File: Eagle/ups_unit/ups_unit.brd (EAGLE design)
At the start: 61 x 20.3 mm, 36 parts

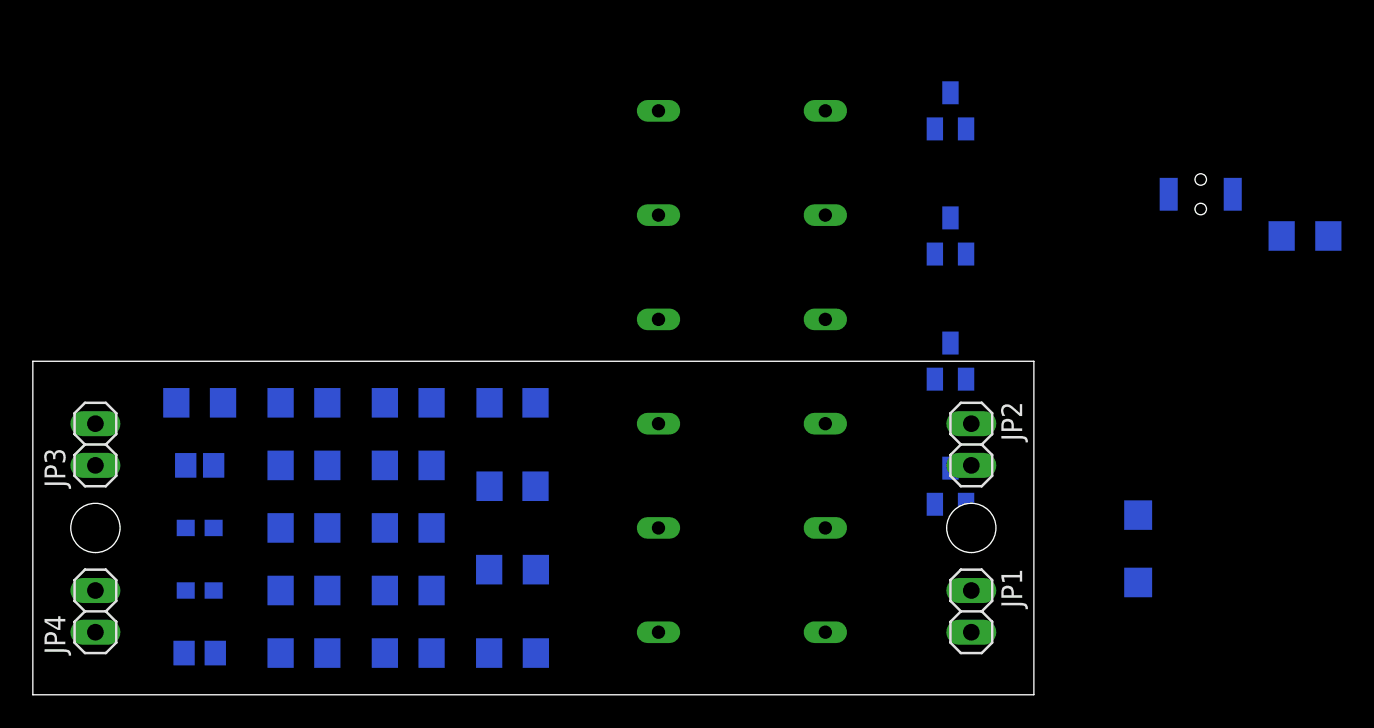
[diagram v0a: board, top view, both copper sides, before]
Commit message: RPi UPS unit
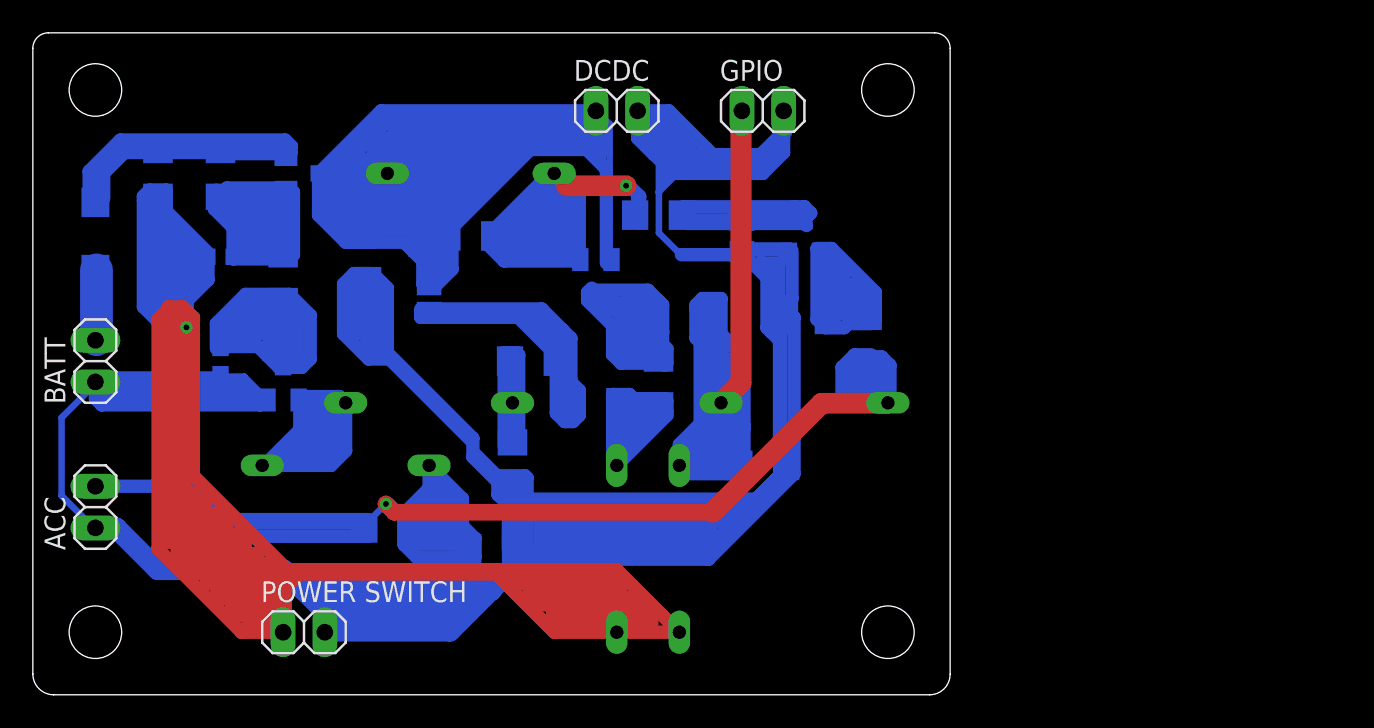
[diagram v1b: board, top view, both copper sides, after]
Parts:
- removed JP1, JP2, JP3, JP4: (no value), pinhead:1X02
- removed S1: MOMENTARY-SWITCH-SPST-SMD-RIGHT-ANGLE, SparkFun-Switches:TACTILE_SWITCH_SMD_RIGHT_ANGLE
- added ACC, BATT, DCDC, GPIO: (no value), pinhead:1X02
- added POWER　SWITCH: (no value), pinhead:1X02
- moved D9 66.3 mm to (3.81, 27.9)
- moved 22UF1 41.7 mm to (43.2, 27.9), turned to 270 degrees
- moved 2N7002K1 40.7 mm to (15.2, 19.1)
- moved DMG3415U2 39.6 mm to (16.5, 31.8), turned to 90 degrees
- moved 3.3K1 36.6 mm to (47.0, 22.9), turned to 180 degrees
- moved D1 32.4 mm to (19.1, 14.0), turned to 180 degrees
- moved 10K3 32.4 mm to (7.62, 31.8), turned to 90 degrees
- moved 5.6K1 29.6 mm to (39.4, 22.9)
- moved 1.8K1 29.0 mm to (44.5, 14.0)
- moved 5.6K2 27.4 mm to (50.8, 21.6), turned to 90 degrees
- moved 10K4 26.8 mm to (15.2, 25.4), turned to 90 degrees
- moved 100K1 24.4 mm to (11.4, 31.8), turned to 90 degrees
- moved DMG3415U1 21.7 mm to (34.3, 25.4), turned to 180 degrees
- moved 100K4 21.6 mm to (38.1, 19.1), turned to 90 degrees
- moved 10K6 21.6 mm to (38.1, 29.2)
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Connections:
- net ACC: now also ACC.2; no longer JP4.2
- net BATT: now also BATT.2; no longer JP3.2
- net DCDC: now also DCDC.1; no longer JP2.1
- net GND: now also ACC.1, BATT.1, DCDC.2, GPIO.2, POWER　SWITCH.2; no longer JP1.2, JP2.2, JP3.1, JP4.1, S1.1
- net GPIO: now also GPIO.1; no longer JP1.1
- net N$104: now also POWER　SWITCH.1; no longer S1.2
- net N$116: now also 10K6.2
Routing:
- net GND: track 0.00 -> 322.7 mm
- net N$104: track 0.00 -> 189.2 mm, vias 0 -> 1
- net DCDC: track 0.00 -> 109.6 mm
- net ACC: track 0.00 -> 85.7 mm, vias 0 -> 1
- net GPIO: track 0.00 -> 62.6 mm
- net N$110: track 0.00 -> 46.8 mm
- net N$116: track 0.00 -> 40.8 mm, vias 0 -> 1
- net N$106: track 0.00 -> 30.5 mm
- net N$103: track 0.00 -> 27.4 mm
- net N$107: track 0.00 -> 26.0 mm
- net N$115: track 0.00 -> 24.8 mm
- net N$113: track 0.00 -> 22.1 mm
- net N$3: track 0.00 -> 21.4 mm
- net N$118: track 0.00 -> 21.3 mm
- net N$108: track 0.00 -> 17.3 mm
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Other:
- board size 61 x 20.3 mm -> 55.9 x 40.3 mm
- board text added: "ACC"
- board text added: "BATT"
- board text added: "DCDCconvertor"
- board text added: "GND"
- board text added: "GPIO"
- board text added: "POWER"
